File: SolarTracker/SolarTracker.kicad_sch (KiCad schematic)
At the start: 1 part, among them U1 ESP32_DevKit_V1_DOIT

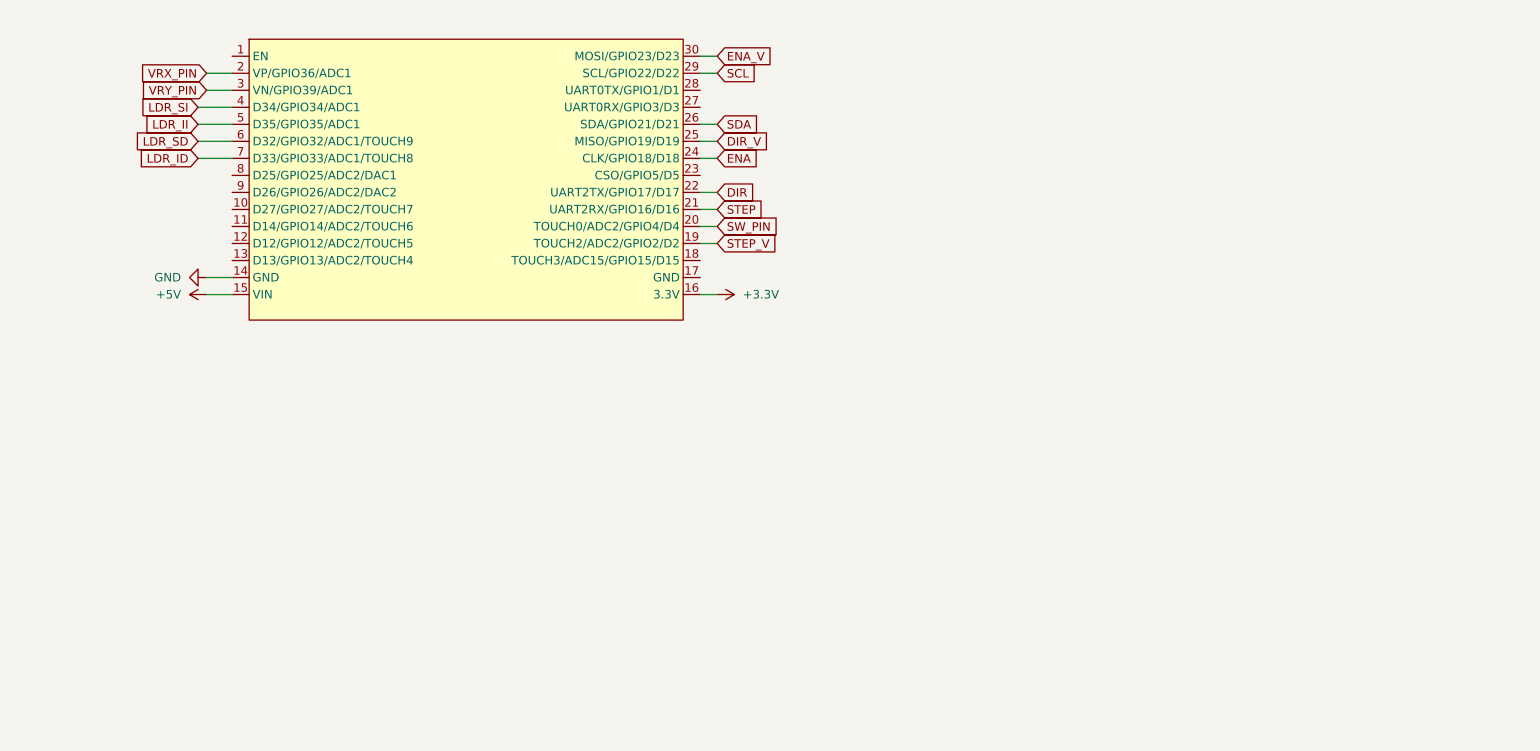
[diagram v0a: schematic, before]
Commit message: PCB Terminadas
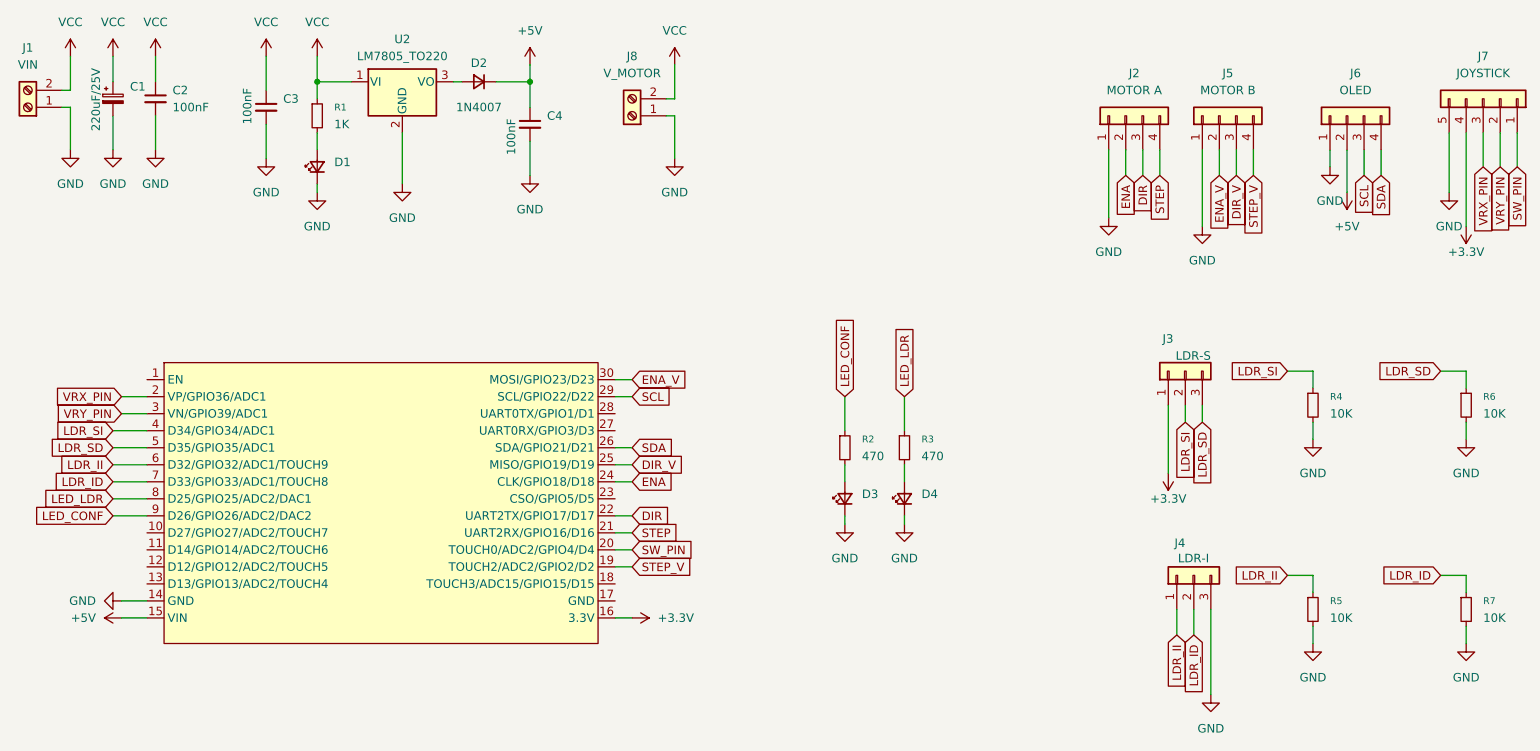
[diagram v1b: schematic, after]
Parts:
- added C1: 220uF/25V, Capacitor_THT:CP_Radial_D6.3mm_P2.50mm, symbol Device:C_Polarized_Small
- added C2, C3, C4: 100nF, Capacitor_THT:C_Disc_D3.8mm_W2.6mm_P2.50mm, symbol Device:C_Small
- added D1, D3, D4: ~, LED_THT:LED_D5.0mm, symbol Device:LED_Small
- added D2: 1N4007, Diode_THT:D_A-405_P10.16mm_Horizontal, symbol Device:D_Small
- added J1: VIN, TerminalBlock_Phoenix:TerminalBlock_Phoenix_MKDS-1,5-2-5.08_1x02_P5.08mm_Horizontal, symbol Connector:Screw_Terminal_01x02
- added J2: MOTOR A, Connector_Molex:Molex_KK-254_AE-6410-04A_1x04_P2.54mm_Vertical, symbol Connector_Generic:Conn_01x04
- added J3: LDR-S, Connector_Molex:Molex_KK-254_AE-6410-03A_1x03_P2.54mm_Vertical, symbol Connector_Generic:Conn_01x03
- added J4: LDR-I, Connector_Molex:Molex_KK-254_AE-6410-03A_1x03_P2.54mm_Vertical, symbol Connector_Generic:Conn_01x03
- added J5: MOTOR B, Connector_Molex:Molex_KK-254_AE-6410-04A_1x04_P2.54mm_Vertical, symbol Connector_Generic:Conn_01x04
- added J6: OLED, Connector_PinSocket_2.54mm:PinSocket_1x04_P2.54mm_Vertical, symbol Connector_Generic:Conn_01x04
- added J7: JOYSTICK, Connector_PinSocket_2.54mm:PinSocket_1x05_P2.54mm_Vertical, symbol Connector_Generic:Conn_01x05
- added J8: V_MOTOR, TerminalBlock_Phoenix:TerminalBlock_Phoenix_MKDS-1,5-2-5.08_1x02_P5.08mm_Horizontal, symbol Connector:Screw_Terminal_01x02
- added R1: 1K, Resistor_THT:R_Axial_DIN0207_L6.3mm_D2.5mm_P10.16mm_Horizontal, symbol Device:R_Small
- added R2, R3: 470, Resistor_THT:R_Axial_DIN0207_L6.3mm_D2.5mm_P10.16mm_Horizontal, symbol Device:R_Small
- added R4, R5, R6, R7: 10K, Resistor_THT:R_Axial_DIN0207_L6.3mm_D2.5mm_P10.16mm_Horizontal, symbol Device:R_Small
- added U2: LM7805_TO220, Package_TO_SOT_THT:TO-220-3_Vertical, symbol Regulator_Linear:LM7805_TO220
- U1: footprint Personal:esp32_devkit_v1_doit -> @EmersonPrez15:ESP32_DEVKIT_V1_E32
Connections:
- net +3.3V: now also J3.1 (Pin_1), J7.4 (Pin_4)
- net +5V: now also C4.1, D2.1 (K), J6.2 (Pin_2)
- net DIR: now also J2.3 (Pin_3)
- net DIR_V: now also J5.3 (Pin_3)
- net ENA: now also J2.2 (Pin_2)
- net ENA_V: now also J5.2 (Pin_2)
- net GND: now also C1.2, C2.2, C3.2, C4.2, D1.1 (K), D3.1 (K), D4.1 (K), J1.1 (Pin_1), J2.1 (Pin_1), J4.3 (Pin_3), J5.1 (Pin_1), J6.1 (Pin_1), J7.5 (Pin_5), J8.1 (Pin_1), R4.2, R5.2, R6.2, R7.2, U2.2 (GND)
- net LDR_ID: now also J4.2 (Pin_2), R7.1
- net LDR_II: now also U1.6 (D32/GPIO32/ADC1/TOUCH9), J4.1 (Pin_1), R5.1; no longer U1.5 (D35/GPIO35/ADC1)
- net LDR_SD: now also U1.5 (D35/GPIO35/ADC1), J3.3 (Pin_3), R6.1; no longer U1.6 (D32/GPIO32/ADC1/TOUCH9)
- net LDR_SI: now also J3.2 (Pin_2), R4.1
- net SCL: now also J6.3 (Pin_3)
- net SDA: now also J6.4 (Pin_4)
- net STEP: now also J2.4 (Pin_4)
- net STEP_V: now also J5.4 (Pin_4)
- net SW_PIN: now also J7.1 (Pin_1)
- net VRX_PIN: now also J7.3 (Pin_3)
- net VRY_PIN: now also J7.2 (Pin_2)
- net LED_LDR: now reaches U1.8 (D25/GPIO25/ADC2/DAC1)
- net LED_LDR: now also R3.1
- net LED_CONF: now reaches U1.9 (D26/GPIO26/ADC2/DAC2)
- net LED_CONF: now also R2.1
- new net: D2.2 (A), U2.3 (VO)
- new net: D3.2 (A), R2.2
- new net: D4.2 (A), R3.2
- new net: D1.2 (A), R1.2
- new net VCC: C1.1, C2.1, C3.1, J1.2 (Pin_2), J8.2 (Pin_2), R1.1, U2.1 (VI)
